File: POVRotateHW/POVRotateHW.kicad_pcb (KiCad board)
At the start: 2 copper layers, 57 parts, among them P1 CONN_01X02, P2 CONN_01X05, U1 A5970AD, U10 APA102C, U11 APA102C, U12 APA102C, U2 M24M01, U3 LMC6062, U4 CYBLE-022001-00, U5 APA102C, U6 APA102C, U7 APA102C, U8 APA102C, U9 APA102C

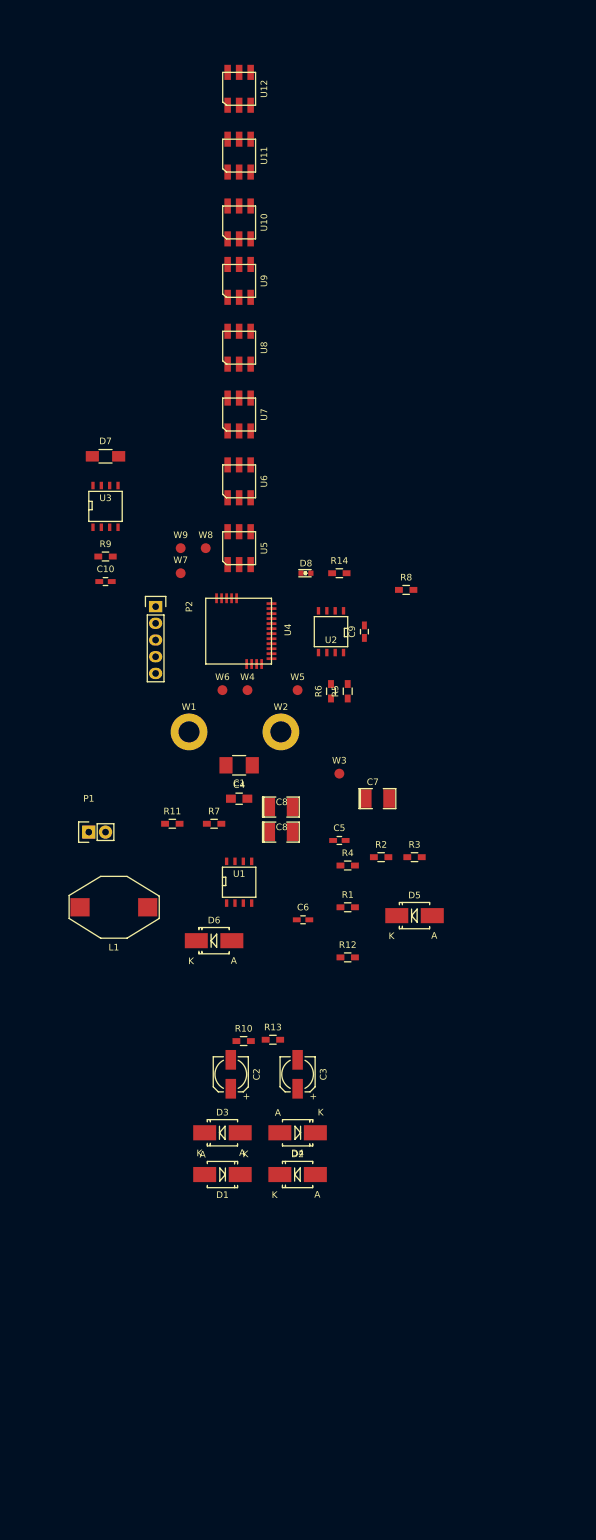
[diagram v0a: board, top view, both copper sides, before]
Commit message: Moved parts around.
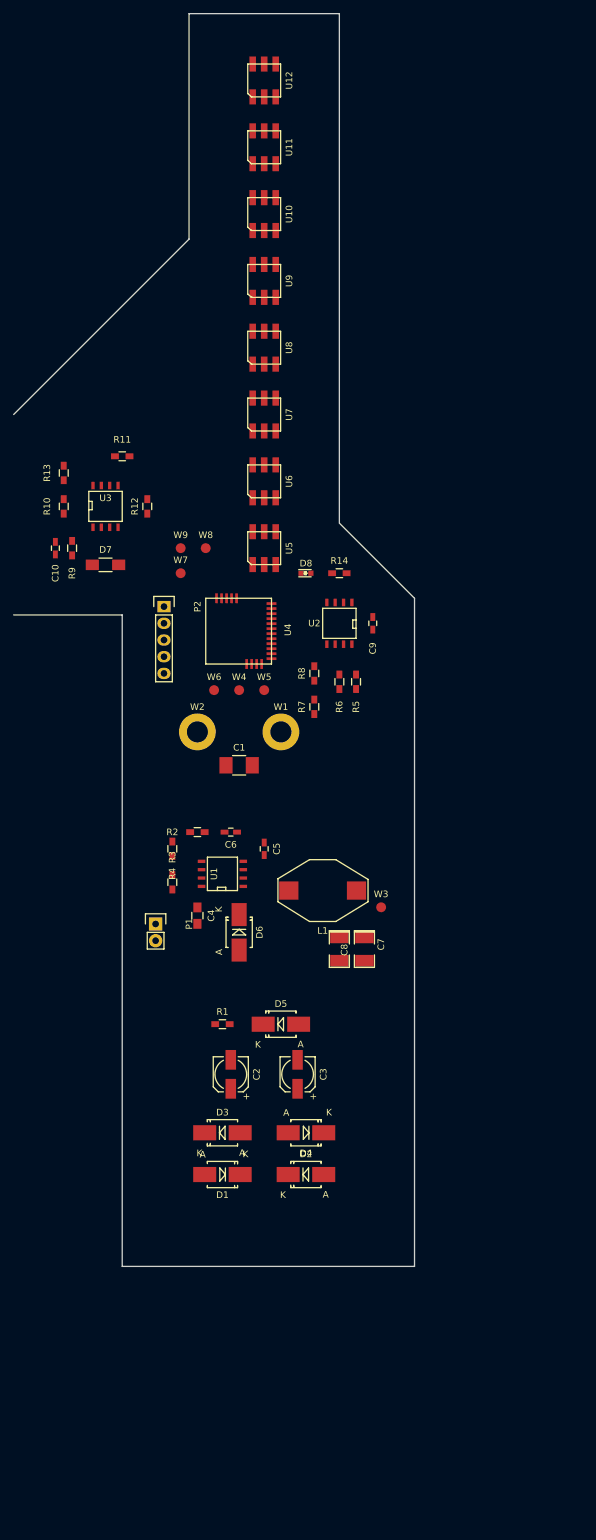
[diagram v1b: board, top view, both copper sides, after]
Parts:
- removed the C8 at (165.1, 138.4)
- moved R13 91.9 mm to (132.1, 83.8), turned to 270 degrees
- moved R10 85.8 mm to (132.1, 88.9), turned to 270 degrees
- moved R12 75.0 mm to (144.8, 88.9), turned to 90 degrees
- moved R11 56.4 mm to (141.0, 81.3), turned to 180 degrees
- moved R3 37.0 mm to (148.6, 146.1), turned to 270 degrees
- moved L1 31.9 mm to (171.4, 147.3)
- moved R2 28.2 mm to (152.4, 138.4), turned to 180 degrees
- moved R4 26.8 mm to (148.6, 141.0), turned to 90 degrees
- moved D5 26.2 mm to (165.1, 167.6)
- moved R1 26.1 mm to (156.2, 167.6)
- moved R7 23.4 mm to (170.2, 119.4), turned to 90 degrees
- moved C8 23.3 mm to (174.0, 156.2), turned to 270 degrees
- moved C7 23.0 mm to (177.8, 156.2), turned to 270 degrees
- moved W3 21.3 mm to (180.3, 149.9)
- moved C4 18.9 mm to (152.4, 151.1), turned to 270 degrees
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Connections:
- P1 pad 1: /Power/12V -> PWR
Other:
- board outline added: 61 x 190.5 mm

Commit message: Working on PCB placement.
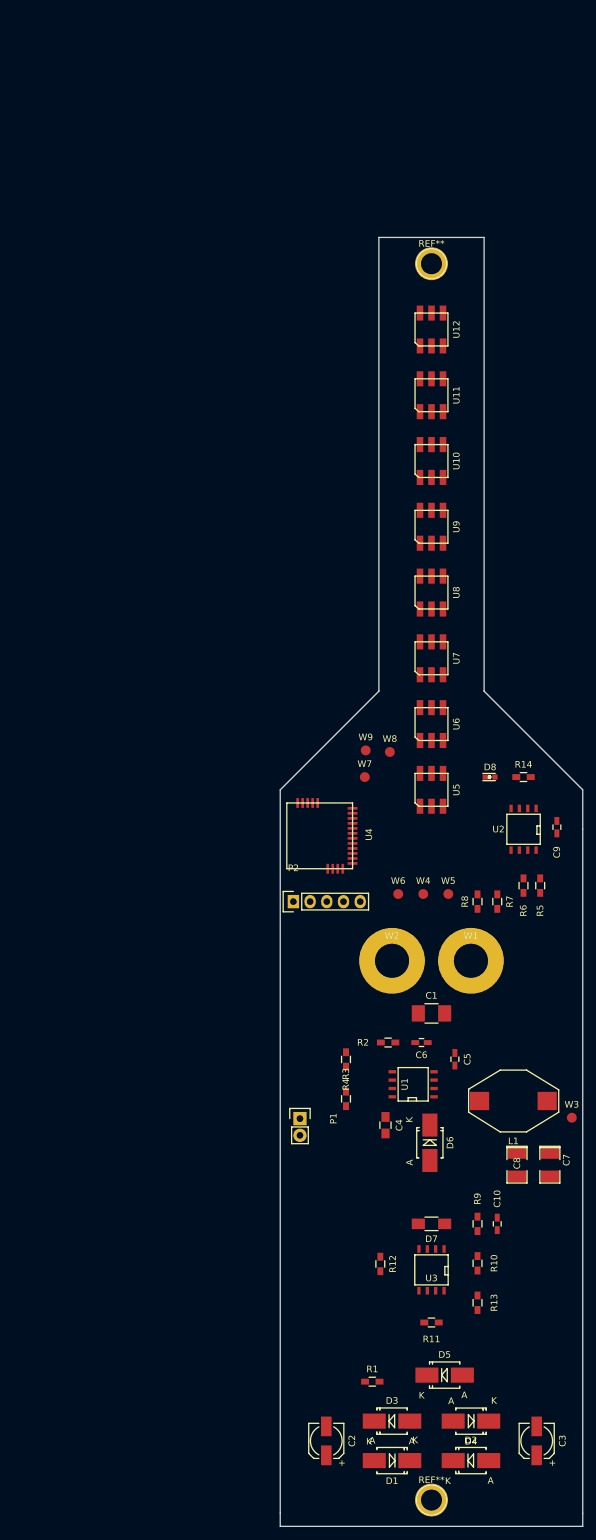
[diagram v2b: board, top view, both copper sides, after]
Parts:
- added REF**: 1pin, Connect:1pin, F.Cu at (188.0, 52.0)
- added REF**: 1pin, Connect:1pin, F.Cu at (188.0, 240.0)
- moved R13 141.0 mm to (195.0, 210.0), turned to 90 degrees
- moved R11 139.9 mm to (188.0, 213.0), turned to 0 degrees
- moved R10 131.2 mm to (195.0, 204.0), turned to 90 degrees
- moved U3 126.2 mm to (188.0, 205.0), turned to 180 degrees
- moved C10 122.8 mm to (198.0, 198.0), turned to 90 degrees
- moved R12 120.5 mm to (180.2, 204.1), turned to 270 degrees
- moved R9 119.8 mm to (195.0, 198.0), turned to 90 degrees
- moved D7 111.8 mm to (188.0, 198.0), turned to 180 degrees
- moved C3 66.6 mm to (204.0, 231.0)
- moved R1 58.9 mm to (179.0, 222.0)
- moved D5 58.9 mm to (190.0, 221.0)
- moved C2 57.6 mm to (172.0, 231.0)
- moved D3 50.9 mm to (182.0, 228.0)
- moved D1 50.6 mm to (182.0, 234.0)
- moved D4 50.5 mm to (194.0, 228.0)
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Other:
- board size 61 x 190.5 mm -> 46 x 196 mm
